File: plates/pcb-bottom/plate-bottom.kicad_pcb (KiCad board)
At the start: 2 copper layers, 152 x 91.6 mm, 9 parts

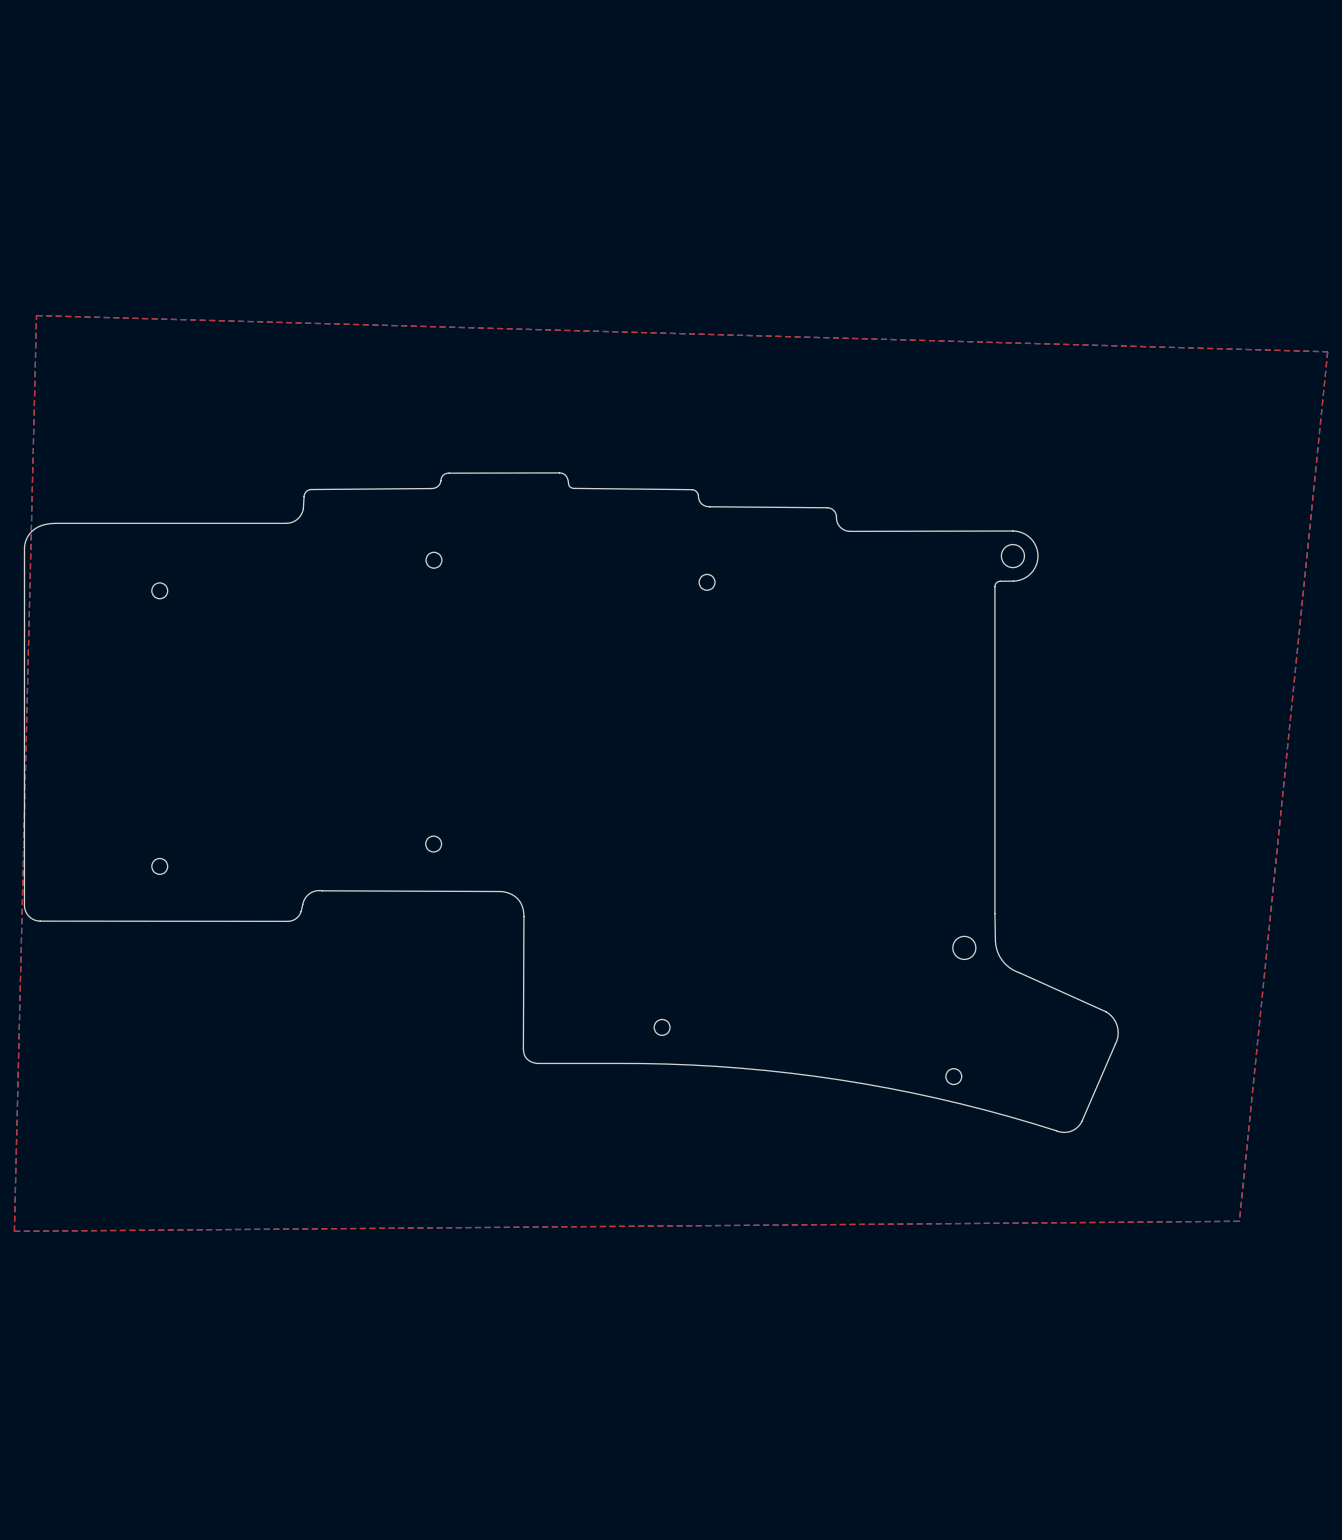
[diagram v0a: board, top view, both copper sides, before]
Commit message: cirrus40, second manufactured version
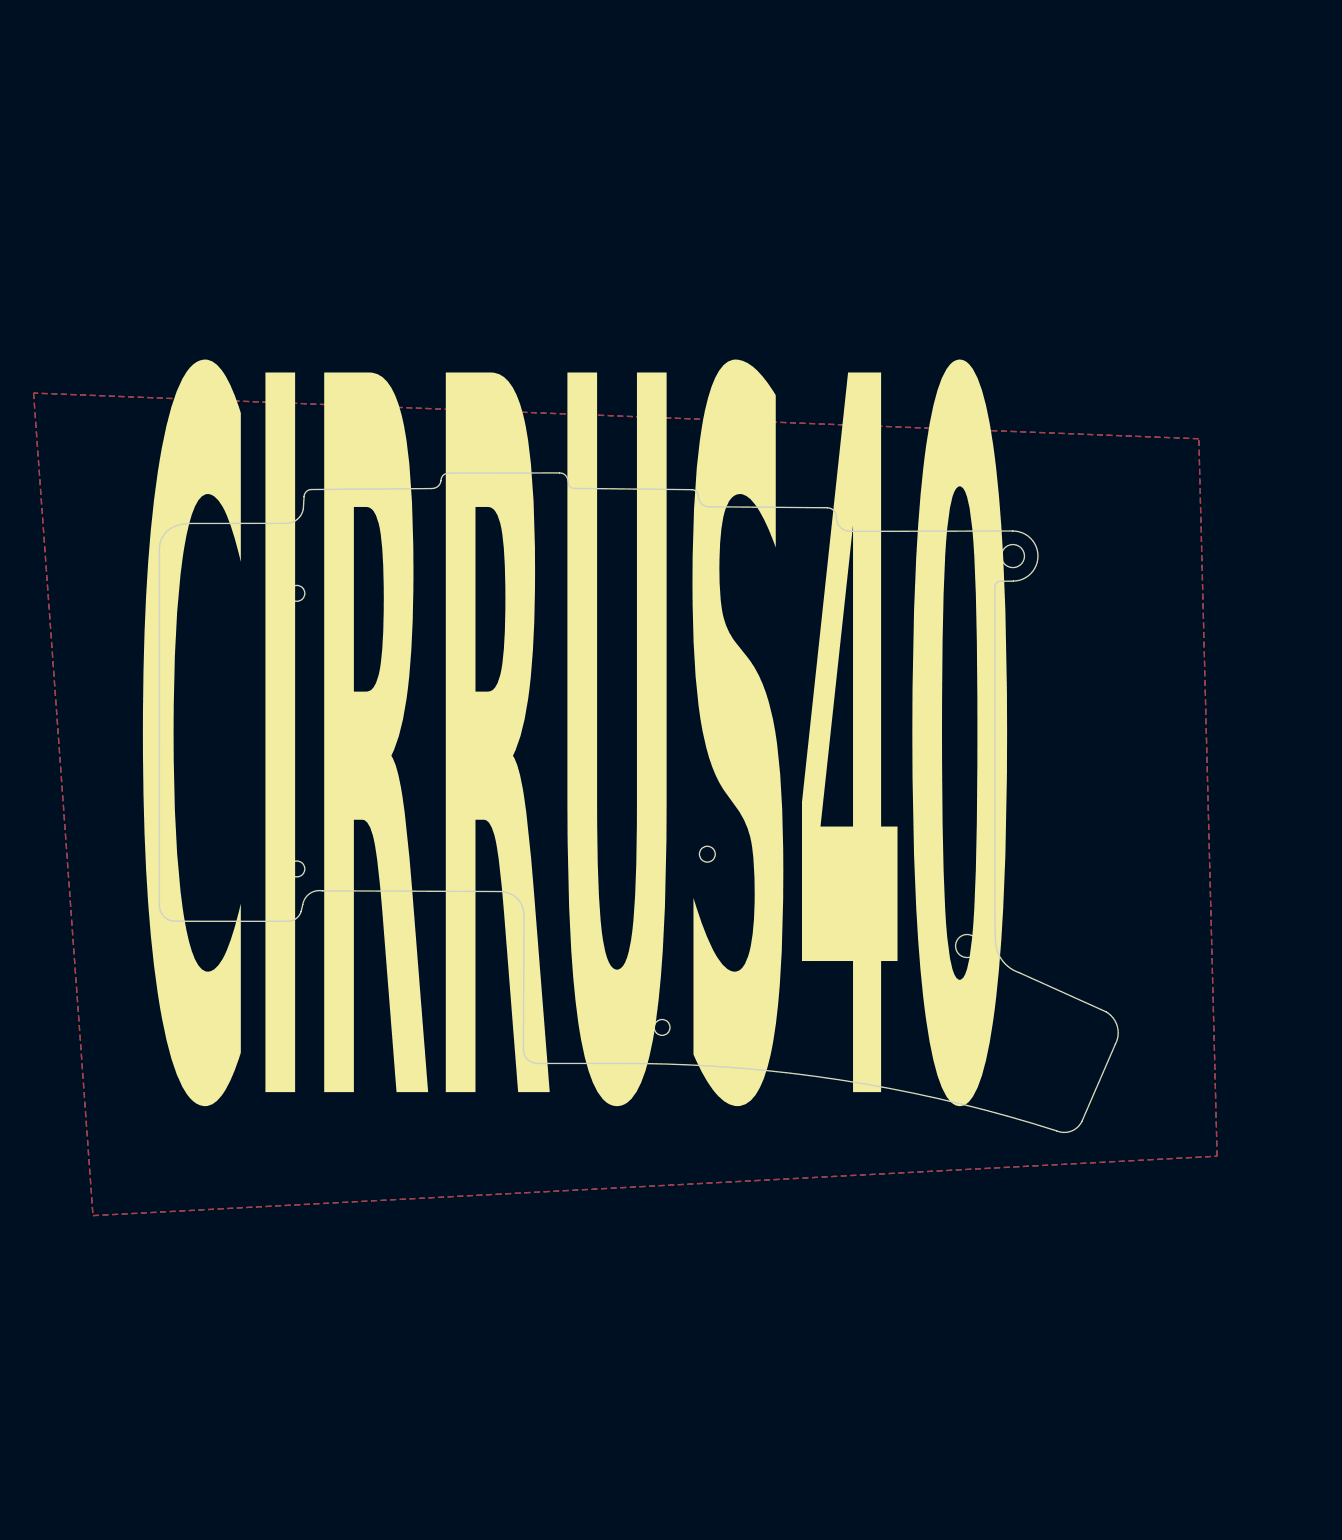
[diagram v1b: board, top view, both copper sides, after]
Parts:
- removed the REF** at (97.5, 61.3)
- moved REF** 38.1 mm to (135.5, 102.2)
- moved REF** 19.1 mm to (78.5, 65.9)
- moved REF** 19.1 mm to (78.5, 104.2)
- moved REF** 1.51 mm to (169.9, 131.6)
- moved REF** 0.46 mm to (171.6, 114.9)
- moved REF** 0.24 mm to (135.5, 64.2)
- renumbered REF** to ?
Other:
- board size 152 x 91.6 mm -> 133.2 x 91.6 mm
- board text added: "CIRRUS40"
